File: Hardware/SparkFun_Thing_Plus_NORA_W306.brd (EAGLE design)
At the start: 22.9 x 58.4 mm, 150 parts, among them J1 THING_PLUS_LOGICAL, J2 LiPo, J3 QWIIC_RA, J4 MICRO-SDFRICTION, J5 USB-C, Q1 3.1A/30V/105mΩ, Q2 MBT3904DW1T1, U1 UBLOX_NORA_W306, U3 XC6222B331MR-G, U4 MCP73831, U5 MAX17048, U6 CP2102N_QFN28

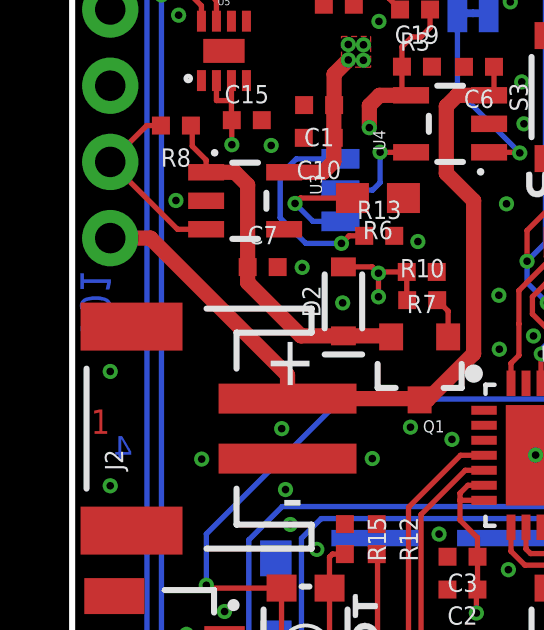
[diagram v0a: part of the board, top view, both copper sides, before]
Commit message: bumping version to v02
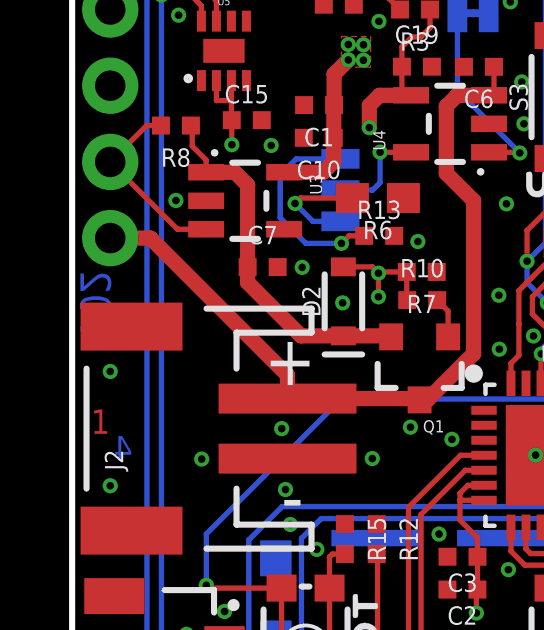
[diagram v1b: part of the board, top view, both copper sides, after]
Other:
- board text added: "v02"
- board text removed: "v01"
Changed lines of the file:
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@@
 <setting verticaltext="up"/>
 </settings>
-<grid distance="0.05" unitdist="inch" unit="inch" style="lines" multiple="1" display="yes" altdistance="0.0001" altunitdist="inch" altunit="inch"/>
+<grid distance="0.05" unitdist="inch" unit="inch" style="lines" multiple="1" display="yes" altdistance="0.005" altunitdist="inch" altunit="inch"/>
 <layers>
 <layer number="1" name="Top" color="4" fill="1" visible="yes" active="yes"/>
@@
 <layer number="20" name="Dimension" color="24" fill="1" visible="yes" active="yes"/>
 <layer number="21" name="tPlace" color="16" fill="1" visible="yes" active="yes"/>
-<layer number="22" name="bPlace" color="14" fill="1" visible="no" active="yes"/>
+<layer number="22" name="bPlace" color="14" fill="1" visible="yes" active="yes"/>
 <layer number="23" name="tOrigins" color="15" fill="1" visible="yes" active="yes"/>
-<layer number="24" name="bOrigins" color="15" fill="1" visible="no" active="yes"/>
+<layer number="24" name="bOrigins" color="15" fill="1" visible="yes" active="yes"/>
 <layer number="25" name="tNames" color="7" fill="1" visible="no" active="yes"/>
 <layer number="26" name="bNames" color="7" fill="1" visible="no" active="yes"/>
@@
 <layer number="48" name="Document" color="7" fill="1" visible="no" active="yes"/>
 <layer number="49" name="Reference" color="7" fill="1" visible="yes" active="yes"/>
-<layer number="51" name="tDocu" color="6" fill="1" visible="no" active="yes"/>
+<layer number="51" name="tDocu" color="6" fill="1" visible="yes" active="yes"/>
 <layer number="52" name="bDocu" color="7" fill="1" visible="no" active="yes"/>
 <layer number="3" name="Route3" color="4" fill="3" visible="no" active="no"/>
@@
 <wire x1="2.54" y1="0" x2="20.32" y2="0" width="0.2032" layer="20"/>
 <wire x1="20.32" y1="0" x2="22.86" y2="2.54" width="0.2032" layer="20" curve="90"/>
-<text x="0.782321875" y="23.0759" size="1.016" layer="16" font="vector" ratio="20" rot="MR270" align="center-left">v01</text>
+<text x="0.782321875" y="23.0759" size="1.016" layer="16" font="vector" ratio="20" rot="MR270" align="center-left">v02</text>
 <text x="0.6223" y="17.604740625" size="0.8128" layer="1" font="vector" ratio="20">1</text>
 <text x="1.3843" y="17.604740625" size="0.8128" layer="2" font="vector" ratio="20">2</text>
